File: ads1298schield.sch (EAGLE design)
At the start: 126 parts, among them IC1 MCP1640SOT23-6-HAND, IC2 ADS1258, J1 22-23-2091, J2 22-23-2091, J3 22-23-2091, Q1 FDD4141TO252, SW3 !RST, U1 MCP73831, U2 LTC3440EMSPBF, X1 SDBMF, X2 USB-MICROB, X3 CRYSTALS-NOGND-91SMX

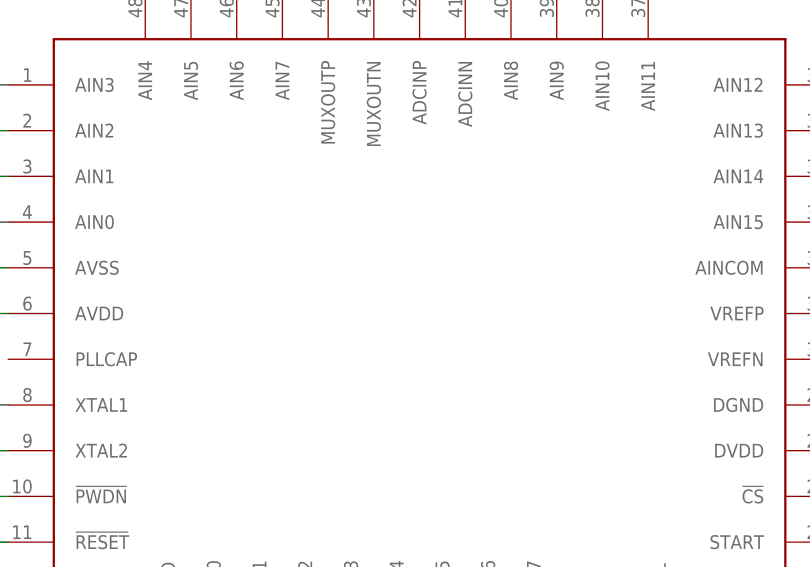
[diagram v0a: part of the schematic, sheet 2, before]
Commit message: v0.4
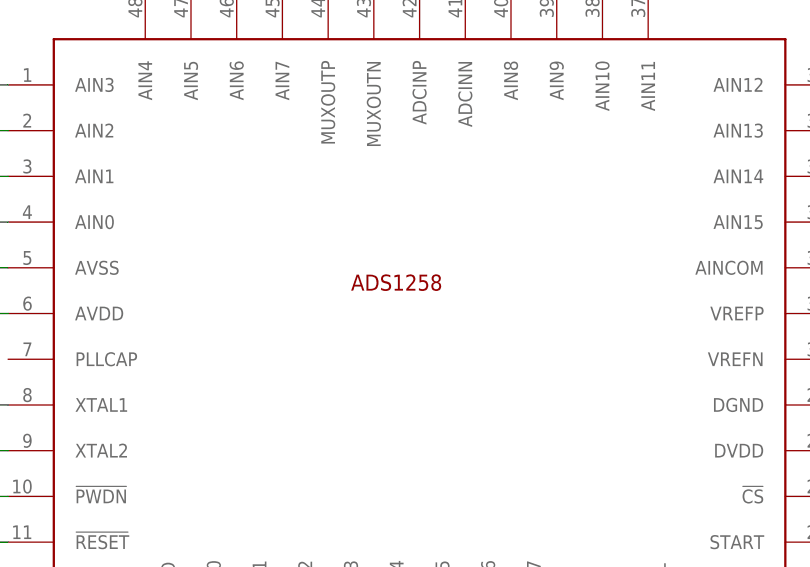
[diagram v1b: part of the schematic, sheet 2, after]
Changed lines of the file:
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@@
 <part name="+3V6" library="supply1" deviceset="+3V3" device=""/>
 <part name="+3V7" library="supply1" deviceset="+3V3" device=""/>
-<part name="FRAME2" library="frames" deviceset="DINA5_L" device=""/>
 <part name="U$3" library="micro-stm_v3" deviceset="STM32F411RE" device=""/>
 <part name="C26" library="rcl" deviceset="C-EU" device="C1210" value="100nF"/>
@@
 <part name="+3V14" library="supply1" deviceset="+3V3" device=""/>
 <part name="SUPPLY54" library="supply2" deviceset="AGND" device=""/>
+<part name="FRAME5" library="frames" deviceset="FRAME_B_L" device=""/>
 </parts>
 <sheets>
@@
 </plain>
 <instances>
-<instance part="FRAME2" gate="G$1" x="-17.78" y="-15.24"/>
 <instance part="U$3" gate="G$1" x="60.96" y="63.5"/>
 <instance part="U$3" gate="G$2" x="134.62" y="45.72"/>
@@
 <instance part="SUPPLY38" gate="G$1" x="-7.62" y="43.18"/>
 <instance part="+3V11" gate="G$1" x="30.48" y="45.72"/>
+<instance part="FRAME5" gate="G$1" x="-66.04" y="-43.18"/>
+<instance part="FRAME5" gate="G$2" x="259.08" y="-43.18"/>
 </instances>
 <busses>
